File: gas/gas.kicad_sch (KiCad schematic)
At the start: 1 part

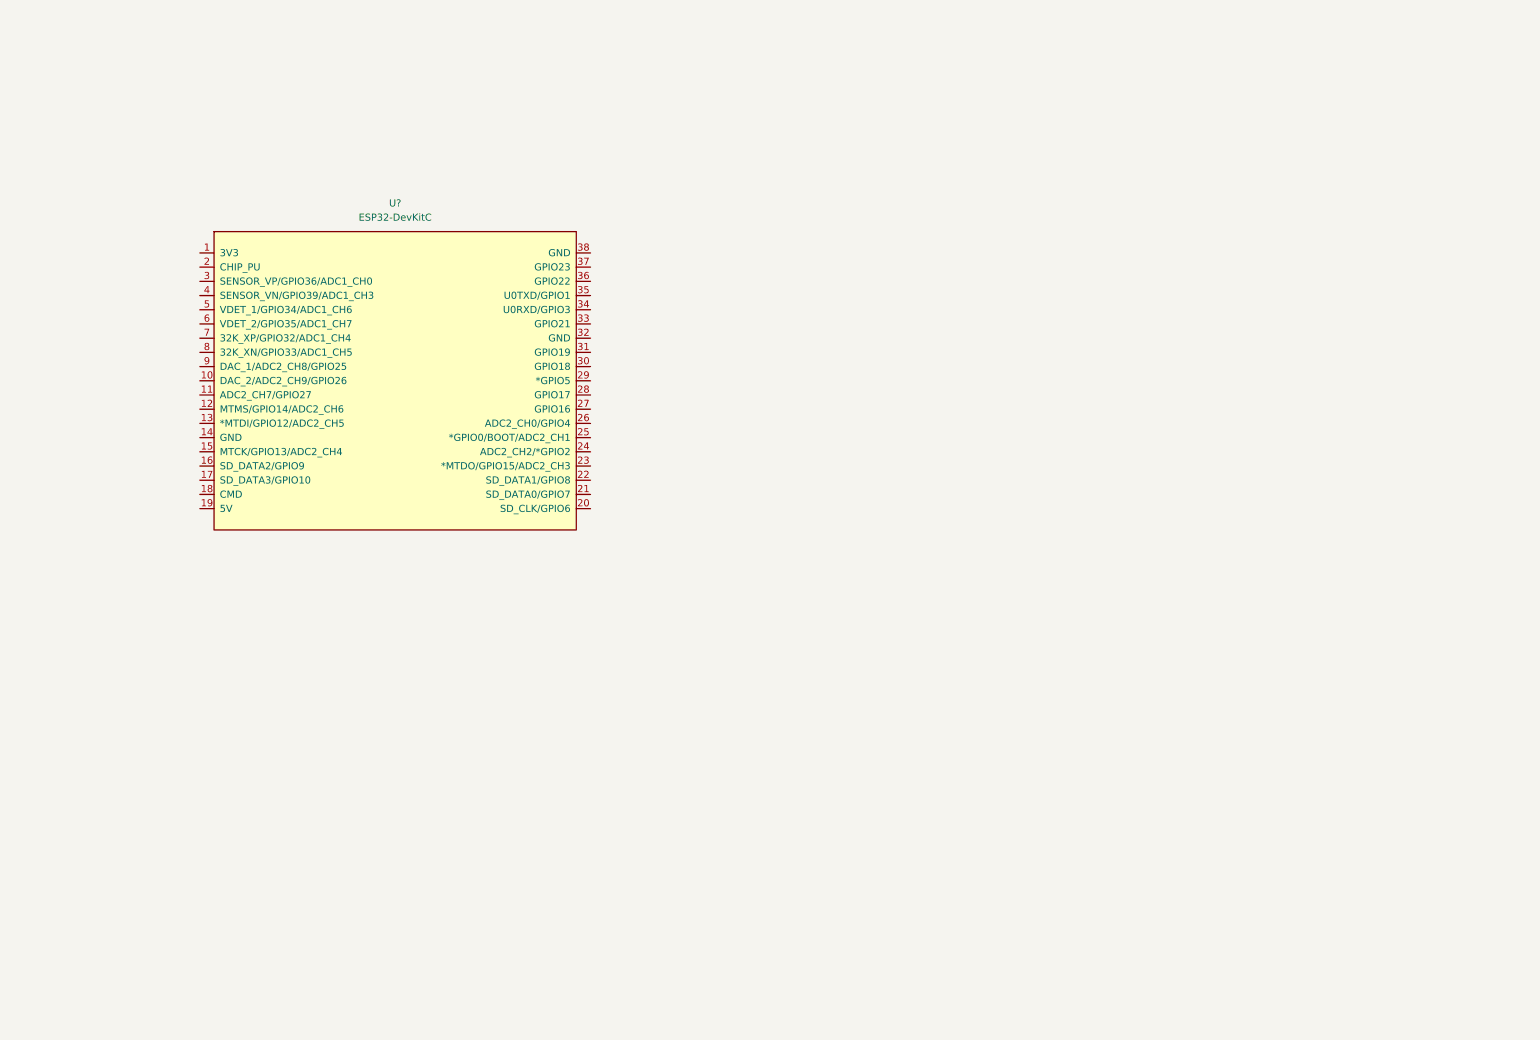
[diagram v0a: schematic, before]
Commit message: basic schema and pcb
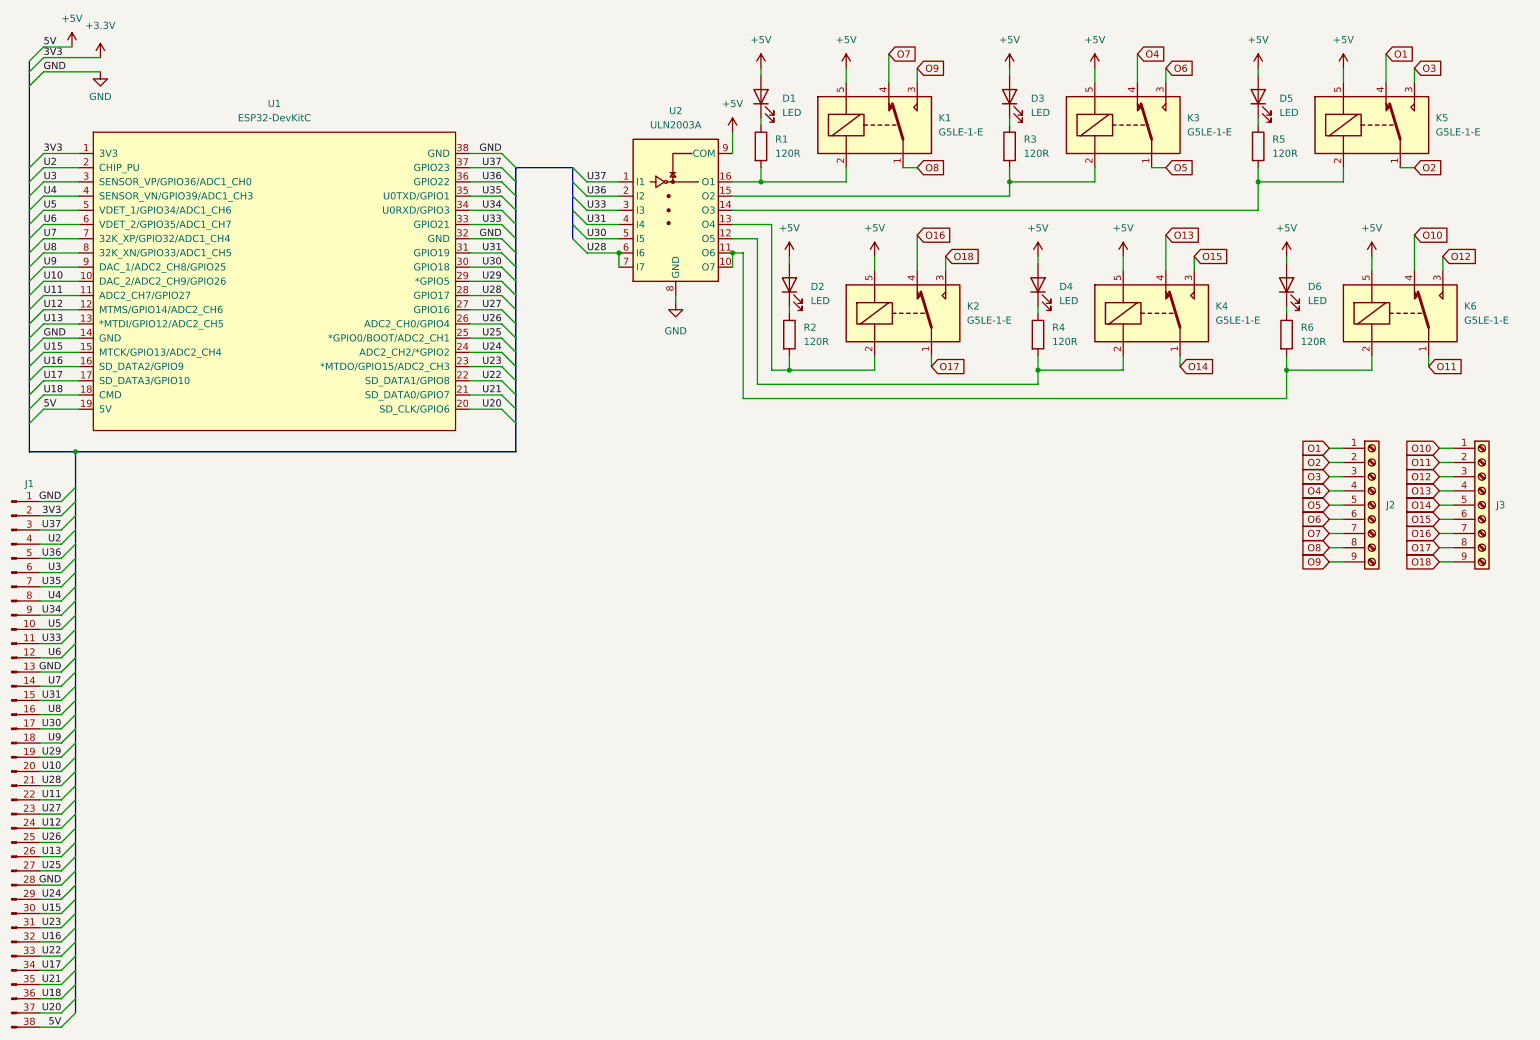
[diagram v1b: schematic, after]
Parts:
- added D1, D2, D3, D4, D5, D6: LED, LED_SMD:LED_0603_1608Metric, symbol Device:LED
- added J1: Conn_01x38_Male, Connector_PinHeader_2.54mm:PinHeader_2x19_P2.54mm_Vertical, symbol Connector:Conn_01x38_Male
- added J2, J3: Screw_Terminal_01x09, TerminalBlock_RND:TerminalBlock_RND_205-00294_1x09_P5.08mm_Horizontal, symbol Connector:Screw_Terminal_01x09
- added K1, K2, K3, K4, K5, K6: G5LE-1-E, Relay_THT:Relay_SPDT_Omron-G5LE-1, symbol Relay:G5LE-1
- added R1, R2, R3, R4, R5, R6: 120R, Resistor_SMD:R_0603_1608Metric, symbol Device:R
- added U2: ULN2003A, Package_SO:SOIC-16_3.9x9.9mm_P1.27mm, symbol Transistor_Array:ULN2003A
- gave numbers to parts that had none: 1
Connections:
- net +3V3: now reaches U1.1 (3V3)
- net +3V3: now also J1.2 (Pin_2)
- net U10: now reaches U1.10 (DAC_2/ADC2_CH9/GPIO26)
- net U10: now also J1.20 (Pin_20)
- net U11: now reaches U1.11 (ADC2_CH7/GPIO27)
- net U11: now also J1.22 (Pin_22)
- net U12: now reaches U1.12 (MTMS/GPIO14/ADC2_CH6)
- net U12: now also J1.24 (Pin_24)
- net U13: now reaches U1.13 (*MTDI/GPIO12/ADC2_CH5)
- net U13: now also J1.26 (Pin_26)
- net GND: now reaches U1.14 (GND)
- net GND: now also U1.32 (GND), U1.38 (GND), J1.1 (Pin_1), J1.13 (Pin_13), J1.28 (Pin_28), U2.8 (GND)
- net U15: now reaches U1.15 (MTCK/GPIO13/ADC2_CH4)
- net U15: now also J1.30 (Pin_30)
- net U16: now reaches U1.16 (SD_DATA2/GPIO9)
- net U16: now also J1.32 (Pin_32)
- net U17: now reaches U1.17 (SD_DATA3/GPIO10)
- net U17: now also J1.34 (Pin_34)
- net U18: now reaches U1.18 (CMD)
- net U18: now also J1.36 (Pin_36)
- net +5V: now reaches U1.19 (5V)
- net +5V: now also D1.2 (A), D2.2 (A), D3.2 (A), D4.2 (A), D5.2 (A), D6.2 (A), J1.38 (Pin_38), K1.5, K2.5, K3.5, K4.5, K5.5, K6.5, U2.9 (COM)
- net U2: now reaches U1.2 (CHIP_PU)
- net U2: now also J1.4 (Pin_4)
- net U20: now reaches U1.20 (SD_CLK/GPIO6)
- net U20: now also J1.37 (Pin_37)
- net U21: now reaches U1.21 (SD_DATA0/GPIO7)
- net U21: now also J1.35 (Pin_35)
- net U22: now reaches U1.22 (SD_DATA1/GPIO8)
- net U22: now also J1.33 (Pin_33)
- net U23: now reaches U1.23 (*MTDO/GPIO15/ADC2_CH3)
- net U23: now also J1.31 (Pin_31)
- net U24: now reaches U1.24 (ADC2_CH2/*GPIO2)
- net U24: now also J1.29 (Pin_29)
- net U25: now reaches U1.25 (*GPIO0/BOOT/ADC2_CH1)
- net U25: now also J1.27 (Pin_27)
- net U26: now reaches U1.26 (ADC2_CH0/GPIO4)
- net U26: now also J1.25 (Pin_25)
- net U27: now reaches U1.27 (GPIO16)
- net U27: now also J1.23 (Pin_23)
- net U28: now reaches U1.28 (GPIO17)
- net U28: now also J1.21 (Pin_21), U2.6 (I6), U2.7 (I7)
- net U29: now reaches U1.29 (*GPIO5)
- net U29: now also J1.19 (Pin_19)
- net U3: now reaches U1.3 (SENSOR_VP/GPIO36/ADC1_CH0)
- net U3: now also J1.6 (Pin_6)
- net U30: now reaches U1.30 (GPIO18)
- net U30: now also J1.17 (Pin_17), U2.5 (I5)
- net U31: now reaches U1.31 (GPIO19)
- net U31: now also J1.15 (Pin_15), U2.4 (I4)
- net U33: now reaches U1.33 (GPIO21)
- net U33: now also J1.11 (Pin_11), U2.3 (I3)
- net U34: now reaches U1.34 (U0RXD/GPIO3)
- net U34: now also J1.9 (Pin_9)
- net U35: now reaches U1.35 (U0TXD/GPIO1)
- net U35: now also J1.7 (Pin_7)
- net U36: now reaches U1.36 (GPIO22)
- net U36: now also J1.5 (Pin_5), U2.2 (I2)
- net U37: now reaches U1.37 (GPIO23)
- net U37: now also J1.3 (Pin_3), U2.1 (I1)
- net U4: now reaches U1.4 (SENSOR_VN/GPIO39/ADC1_CH3)
- net U4: now also J1.8 (Pin_8)
- net U5: now reaches U1.5 (VDET_1/GPIO34/ADC1_CH6)
- net U5: now also J1.10 (Pin_10)
- net U6: now reaches U1.6 (VDET_2/GPIO35/ADC1_CH7)
- net U6: now also J1.12 (Pin_12)
- net U7: now reaches U1.7 (32K_XP/GPIO32/ADC1_CH4)
- net U7: now also J1.14 (Pin_14)
- net U8: now reaches U1.8 (32K_XN/GPIO33/ADC1_CH5)
- net U8: now also J1.16 (Pin_16)
- net U9: now reaches U1.9 (DAC_1/ADC2_CH8/GPIO25)
- net U9: now also J1.18 (Pin_18)
- new net: D4.1 (K), R4.1
- new net: K4.2, R4.2, U2.12 (O5)
- new net: D5.1 (K), R5.1
- new net: K5.2, R5.2, U2.14 (O3)
- new net: K2.2, R2.2, U2.13 (O4)
- new net: D6.1 (K), R6.1
- new net: K6.2, R6.2, U2.10 (O7), U2.11 (O6)
- new net: K3.2, R3.2, U2.15 (O2)
- new net: K1.2, R1.2, U2.16 (O1)
- new net: D1.1 (K), R1.1
- new net: D2.1 (K), R2.1
- new net: D3.1 (K), R3.1
- new net O1: J2.1 (Pin_1), K5.4
- new net O10: J3.1 (Pin_1), K6.4
- new net O11: J3.2 (Pin_2), K6.1
- new net O12: J3.3 (Pin_3), K6.3
- new net O13: J3.4 (Pin_4), K4.4
- new net O14: J3.5 (Pin_5), K4.1
- new net O15: J3.6 (Pin_6), K4.3
- new net O16: J3.7 (Pin_7), K2.4
- new net O17: J3.8 (Pin_8), K2.1
- new net O18: J3.9 (Pin_9), K2.3
- new net O2: J2.2 (Pin_2), K5.1
- new net O3: J2.3 (Pin_3), K5.3
- new net O4: J2.4 (Pin_4), K3.4
- new net O5: J2.5 (Pin_5), K3.1
- new net O6: J2.6 (Pin_6), K3.3
- new net O7: J2.7 (Pin_7), K1.4
- new net O8: J2.8 (Pin_8), K1.1
- new net O9: J2.9 (Pin_9), K1.3
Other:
- moved on the sheet: U1
